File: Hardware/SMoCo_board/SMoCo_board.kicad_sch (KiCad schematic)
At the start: 43 parts, among them J1 Conn_01x02, J2 Conn_01x02, J3 Conn_01x03, J5 Conn_01x06, J6 Conn_01x02, J7 Conn_01x04, J8 Conn_01x02, SW1 SW_Push, U1 STM32F072C8T6, U2 VNH7040AYTR, U3 SN65HVD232, U4 AP63203WU

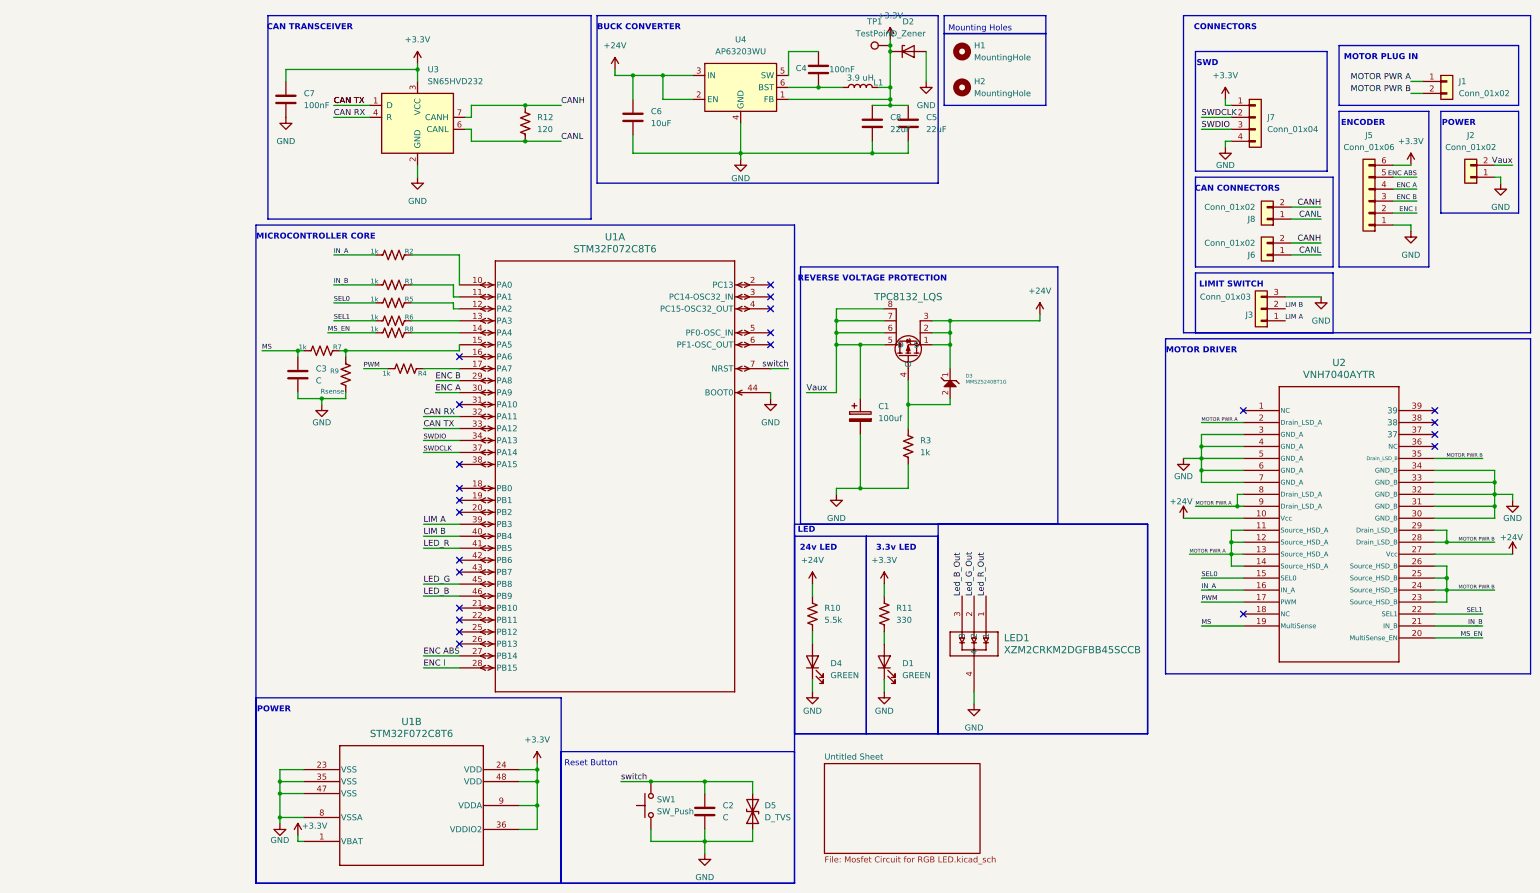
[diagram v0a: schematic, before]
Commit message: Temp Revision SMoCo
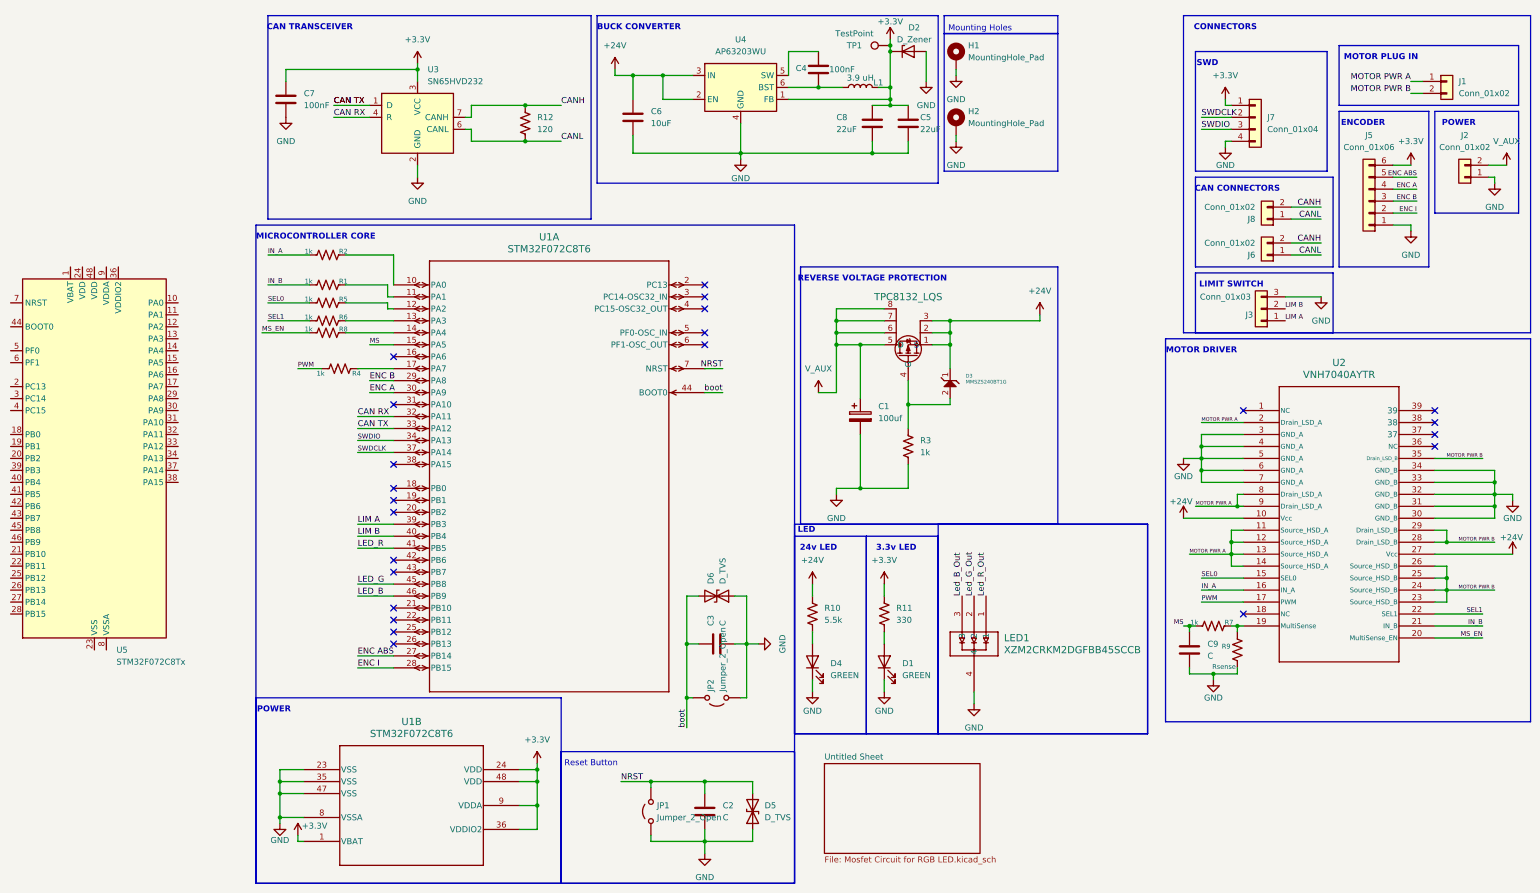
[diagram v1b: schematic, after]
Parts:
- removed H1, H2: MountingHole, symbol Mechanical:MountingHole
- removed SW1: SW_Push, Button_Switch_SMD:Nidec_Copal_CAS-120A, symbol Switch:SW_Push
- added C9: C, symbol Device:C
- added D6: D_TVS, Diode_SMD:D_0603_1608Metric_Pad1.05x0.95mm_HandSolder, symbol Device:D_TVS
- added H1, H2: MountingHole_Pad, symbol Mechanical:MountingHole_Pad
- added JP1, JP2: Jumper_2_Open, Package_LCC:PLCC-84_29.3x29.3mm_P1.27mm, symbol Jumper:Jumper_2_Open
- added U5: STM32F072C8Tx, Package_QFP:LQFP-48_7x7mm_P0.5mm, symbol MCU_ST_STM32F0:STM32F072C8Tx
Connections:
- net GND: now also C9.2, D6.1 (A1), H1.1, H2.1, JP1.1 (A), JP2.1 (A); no longer U1.44 (BOOT0)
- net MS: now also U1.15 (PA5), C9.1; no longer C3.1, U2.19 (MultiSense)
- net at R7.2, R9.1: now also U2.19 (MultiSense); no longer U1.15 (PA5)
- net Vaux renamed V_AUX
- net switch renamed NRST
- net NRST: now also JP1.2 (B)
- new net: U5.23 (VSS), U5.35 (VSS), U5.47 (VSS)
- new net boot: C3.1, D6.2 (A2), JP2.2 (B), U1.44 (BOOT0)
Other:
- moved on the sheet: J2, R1, R2, R4, R5, R6, R8, U1A
